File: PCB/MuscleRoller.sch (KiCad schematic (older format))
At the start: 28 parts, among them J1 Screw_Terminal_01x02, J10 Conn_01x04_Male, J11 Conn_01x03_Male, J12 Conn_01x03_Male, J2 Conn_02x03_Odd_Even, J3 Conn_02x03_Odd_Even, J4 Conn_01x04_Male, J5 Conn_01x04_Male, J6 Conn_01x03_Male, J7 Conn_01x04_Male, J8 Conn_01x04_Male, J9 Conn_01x04_Male, U1 AZ1117-3.3, U2 ESP32-S2-WROOM

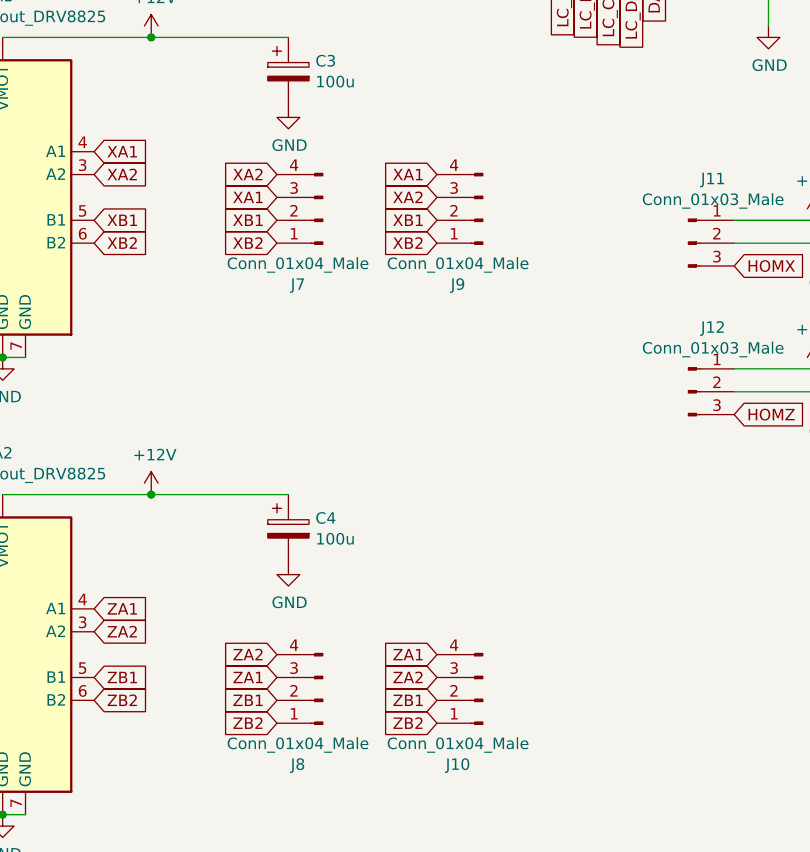
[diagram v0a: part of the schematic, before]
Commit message: PCB order
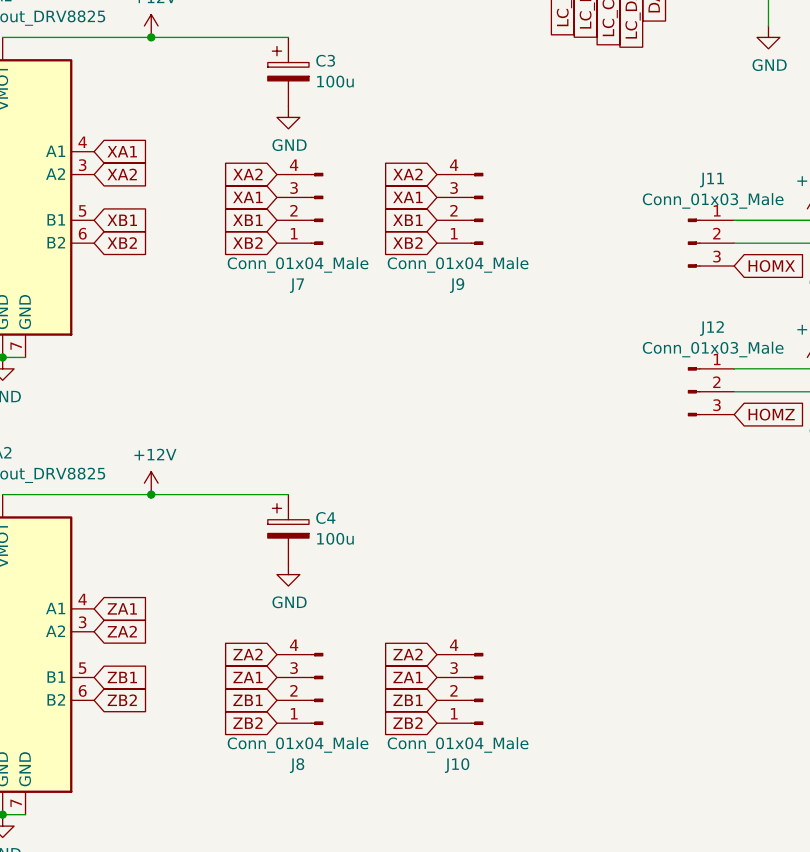
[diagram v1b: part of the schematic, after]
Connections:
- net XA1: now also J9.3 (Pin_3); no longer J9.4 (Pin_4)
- net XA2: now also J9.4 (Pin_4); no longer J9.3 (Pin_3)
- net ZA1: now also J10.3 (Pin_3); no longer J10.4 (Pin_4)
- net ZA2: now also J10.4 (Pin_4); no longer J10.3 (Pin_3)
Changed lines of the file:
@@
 Text GLabel 3850 4900 0    50   Input ~ 0
 XB2
+Text GLabel 4550 4700 0    50   Input ~ 0
+XA1
 Text GLabel 4550 4600 0    50   Input ~ 0
-XA1
-Text GLabel 4550 4700 0    50   Input ~ 0
 XA2
 Text GLabel 4550 4800 0    50   Input ~ 0
@@
 Text GLabel 3850 7000 0    50   Input ~ 0
 ZB2
+Text GLabel 4550 6800 0    50   Input ~ 0
+ZA1
 Text GLabel 4550 6700 0    50   Input ~ 0
-ZA1
-Text GLabel 4550 6800 0    50   Input ~ 0
 ZA2
 Text GLabel 4550 6900 0    50   Input ~ 0
